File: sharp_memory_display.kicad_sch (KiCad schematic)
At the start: 16 parts, among them J1 Conn_01x05, J2 Conn_01x10, J3 Conn_01x05_Male, J4 Conn_01x10

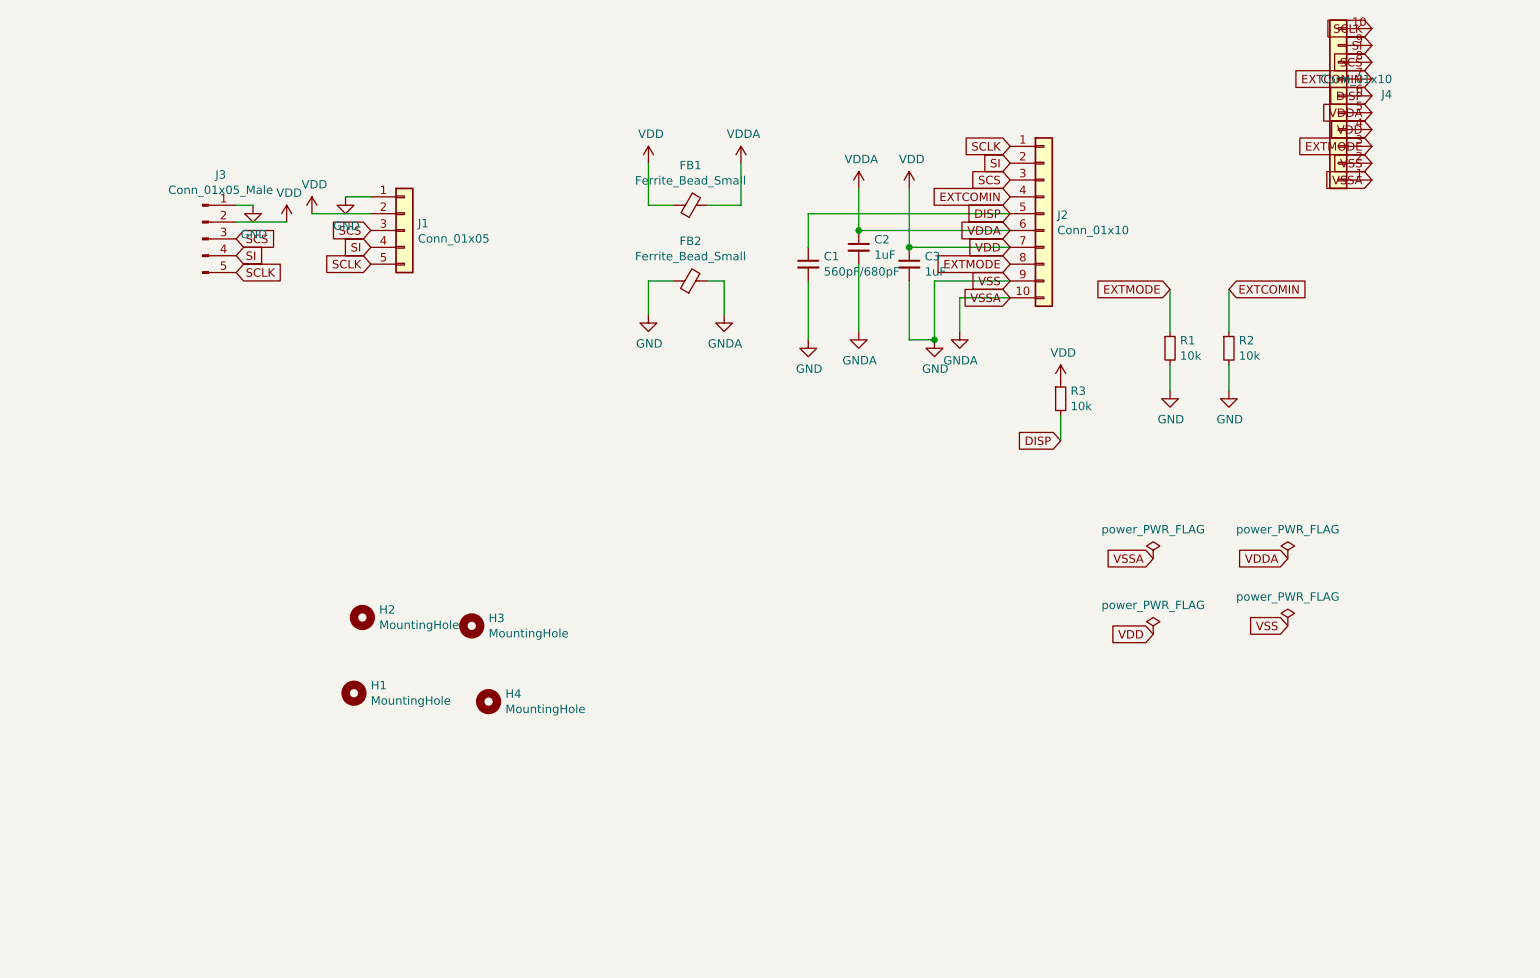
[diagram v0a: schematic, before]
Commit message: tidy up schematic
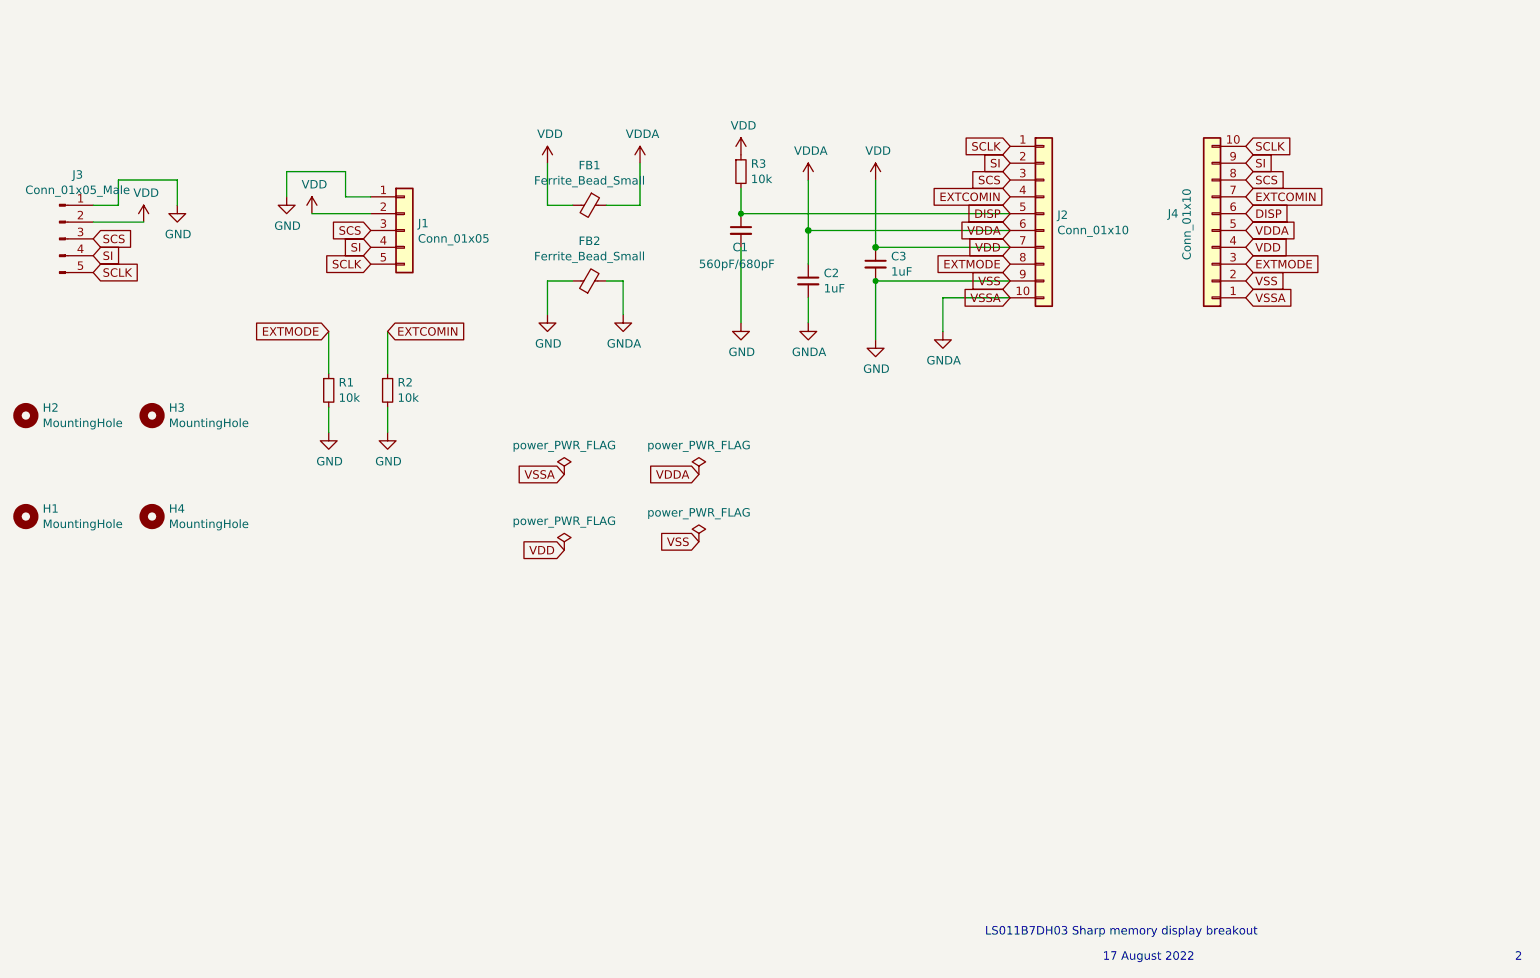
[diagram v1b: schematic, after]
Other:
- note added: "17 August 2022"
- note added: "2"
- note added: "LS011B7DH03 Sharp memory display breakout"
- moved on the sheet: C1, C2, C3, FB1, FB2, H1, H2, H3, H4, J3, J4, R1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
